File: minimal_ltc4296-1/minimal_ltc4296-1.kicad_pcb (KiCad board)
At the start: 4 copper layers, 50.8 x 30.5 mm, 38 parts, among them Q1 100.0 V, Q2 100.0 V, Q3 100.0 V, Q4 100.0 V, Q5 100.0 V, Q6 100.0 V, U1 LTC4296AUK-1-PBF

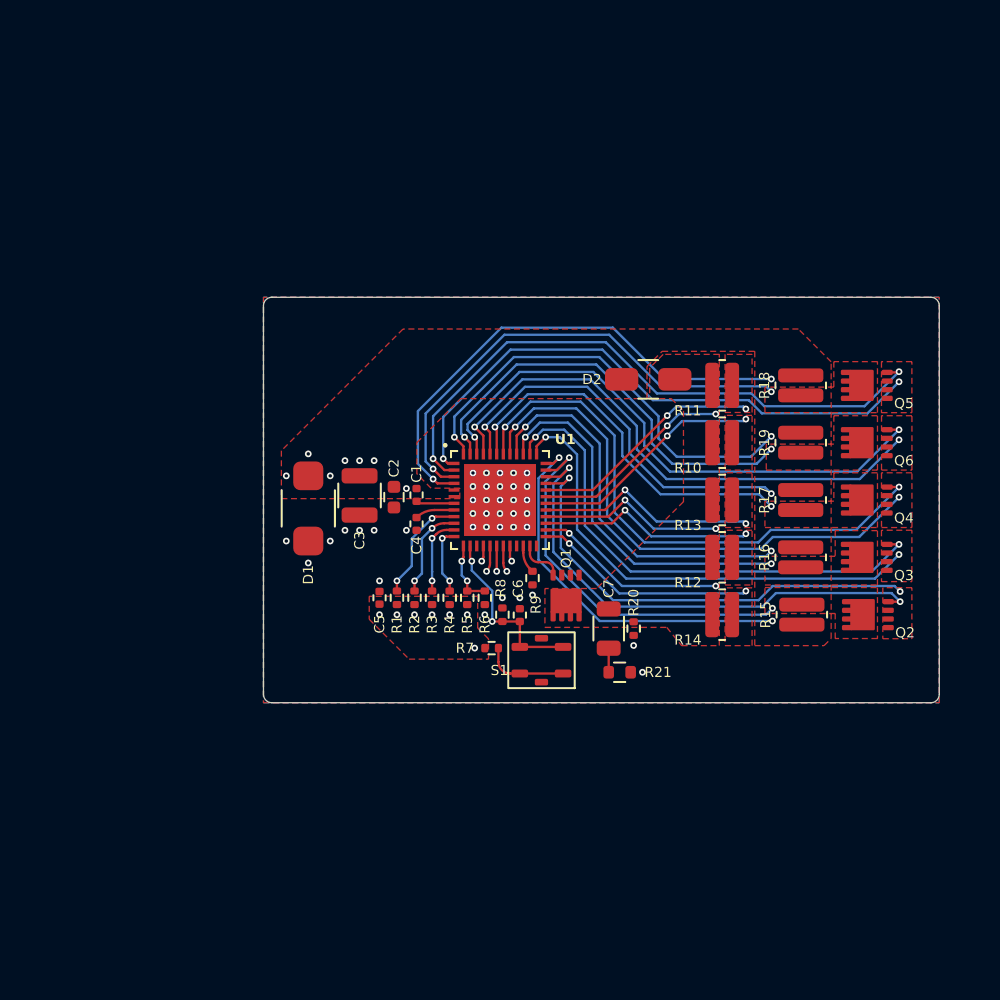
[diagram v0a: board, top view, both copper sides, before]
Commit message: Update PCB layout and schematic
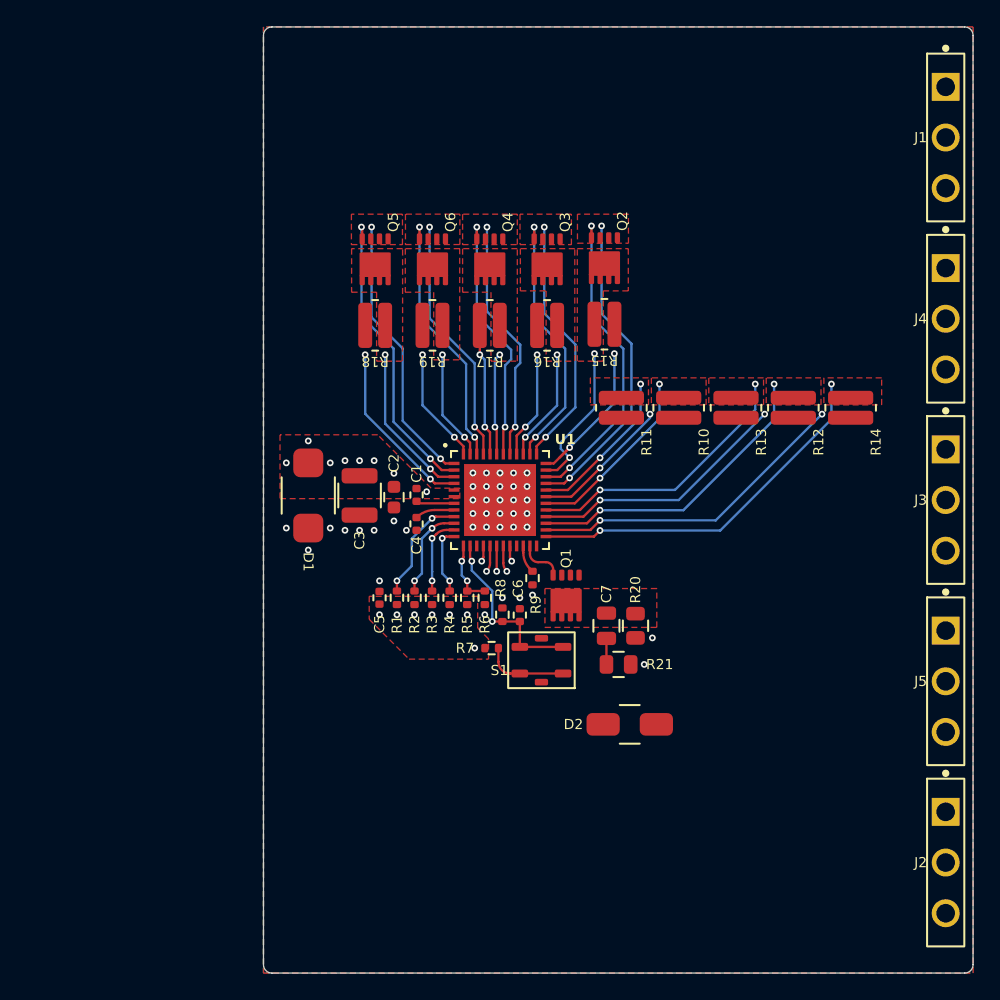
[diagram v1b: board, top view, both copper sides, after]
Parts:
- added J1: TBP02R1-381-03BE, connector_footprints:TBP02R1-381-03BE, F.Cu at (183.2, 75.1)
- added J2: TBP02R1-381-03BE, connector_footprints:TBP02R1-381-03BE, F.Cu at (183.2, 129.6)
- added J3: TBP02R1-381-03BE, connector_footprints:TBP02R1-381-03BE, F.Cu at (183.2, 102.4)
- added J4: TBP02R1-381-03BE, connector_footprints:TBP02R1-381-03BE, F.Cu at (183.2, 88.7)
- added J5: TBP02R1-381-03BE, connector_footprints:TBP02R1-381-03BE, F.Cu at (183.2, 116.0)
- C7: footprint capacitor_footprints:C_1206_3216Metric -> capacitor_footprints:C_0805_2012Metric
- R20: footprint resistor_footprints:R_0402_1005Metric -> resistor_footprints:R_0805_2012Metric
- R21: footprint resistor_footprints:R_0603_1608Metric -> resistor_footprints:R_0805_2012Metric
- moved Q5 38.2 mm to (140.3, 84.3), turned to -90 degrees
- moved Q6 35.4 mm to (144.6, 84.3), turned to -90 degrees
- moved Q4 33.6 mm to (148.9, 84.3), turned to -90 degrees
- moved Q2 33.3 mm to (157.6, 84.2), turned to -90 degrees
- moved Q3 32.8 mm to (153.2, 84.3), turned to -90 degrees
- moved R18 32.3 mm to (140.3, 89.2), turned to 0 degrees
- moved R19 29.1 mm to (144.6, 89.2), turned to 0 degrees
- moved R17 26.8 mm to (148.9, 89.2), turned to 0 degrees
- moved R15 26.4 mm to (157.6, 89.1), turned to 180 degrees
- moved D2 26.0 mm to (159.5, 119.2)
- moved R16 25.8 mm to (153.2, 89.2), turned to 0 degrees
- moved R14 18.3 mm to (176.1, 95.4), turned to 90 degrees
- moved R12 12.5 mm to (171.8, 95.4), turned to 90 degrees
- moved R11 7.76 mm to (158.8, 95.4), turned to 90 degrees
- moved R13 7.01 mm to (167.4, 95.4), turned to 90 degrees
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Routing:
- net /PSE: track 159.4 -> 51.9 mm, vias 17 -> 18
- net /HSNSM0: track 36.4 -> 12.0 mm
- net /HSNSM1: track 32.5 -> 8.33 mm
- net /HGATE0: track 46.4 -> 22.6 mm
- net /HGATE2: track 42.9 -> 19.3 mm
- net /HGATE1: track 42.9 -> 19.7 mm
- net /OUTP0: track 43.4 -> 20.7 mm
- net /OUTP2: track 41.0 -> 18.4 mm
- net /OUTP1: track 41.0 -> 18.7 mm
- net /HSNSM2: track 28.4 -> 7.67 mm
- net /HSNSM3: track 28.0 -> 8.52 mm
- net /HGATE3: track 38.5 -> 20.0 mm
- net /HSNSM4: track 29.3 -> 11.3 mm
- net /OUTP3: track 36.6 -> 19.2 mm
- net /HGATE4: track 38.2 -> 23.8 mm
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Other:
- board size 50.8 x 30.5 mm -> 53.3 x 71.1 mm

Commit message: Update PCB layout
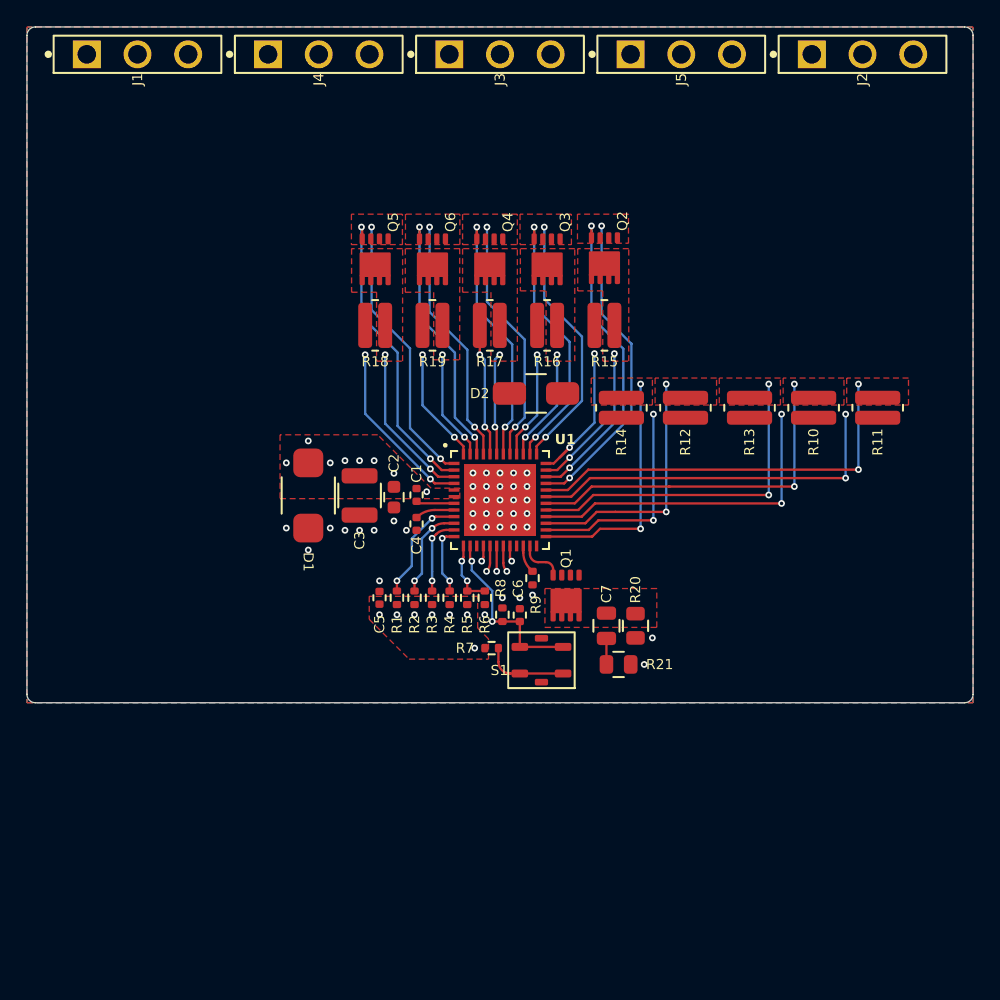
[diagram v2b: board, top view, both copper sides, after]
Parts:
- moved J2 61.1 mm to (177.0, 68.9), turned to 0 degrees
- moved J1 61.1 mm to (122.5, 68.9), turned to 0 degrees
- moved J5 51.1 mm to (163.3, 68.9), turned to 0 degrees
- moved J4 51.1 mm to (136.1, 68.9), turned to 0 degrees
- moved J3 47.4 mm to (149.7, 68.9), turned to 0 degrees
- moved D2 25.9 mm to (152.4, 94.4)
- moved R11 19.3 mm to (178.1, 95.4)
- moved R14 17.2 mm to (158.8, 95.4)
- moved R10 10.1 mm to (173.3, 95.4)
- moved R12 8.11 mm to (163.6, 95.4)
- moved R13 1.02 mm to (168.5, 95.4)
- moved R15 0.09 mm to (157.6, 89.2), turned to 0 degrees
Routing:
- net /OUTM4: track 11.9 -> 30.6 mm
- net /LSNS: track 54.6 -> 69.1 mm
- net /OUTM3: track 13.8 -> 26.9 mm
- net /OUTM0: track 27.8 -> 18.2 mm
- net /OUTM2: track 20.8 -> 25.6 mm
- net /OUTM1: track 23.0 -> 19.0 mm
- net /PSE: track 51.9 -> 51.3 mm
- removed copper zone on In1.Cu, net /LSNS
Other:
- board size 53.3 x 71.1 mm -> 71.1 x 50.8 mm
